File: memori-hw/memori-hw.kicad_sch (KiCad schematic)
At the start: 3 parts, among them J1 Conn_02x04_Odd_Even, J2 Conn_01x07, J3 Conn_01x07

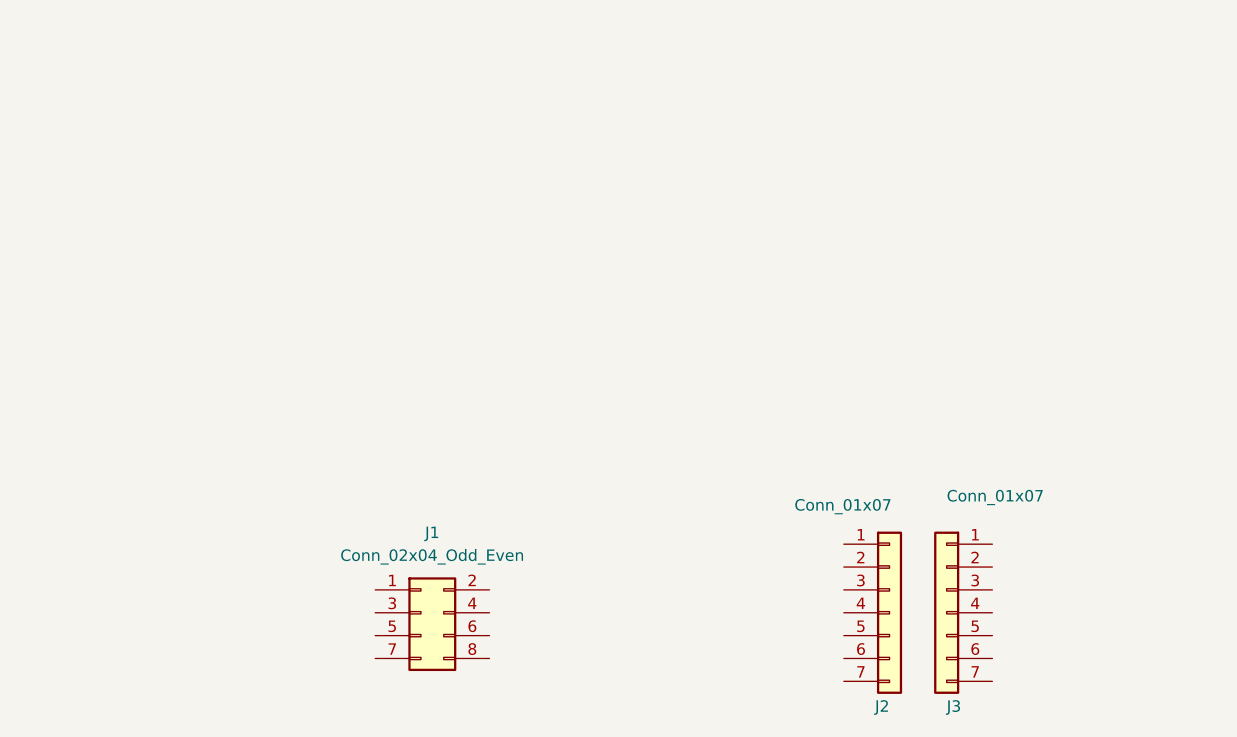
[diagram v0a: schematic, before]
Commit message: feat(hw): Finished with schematic.
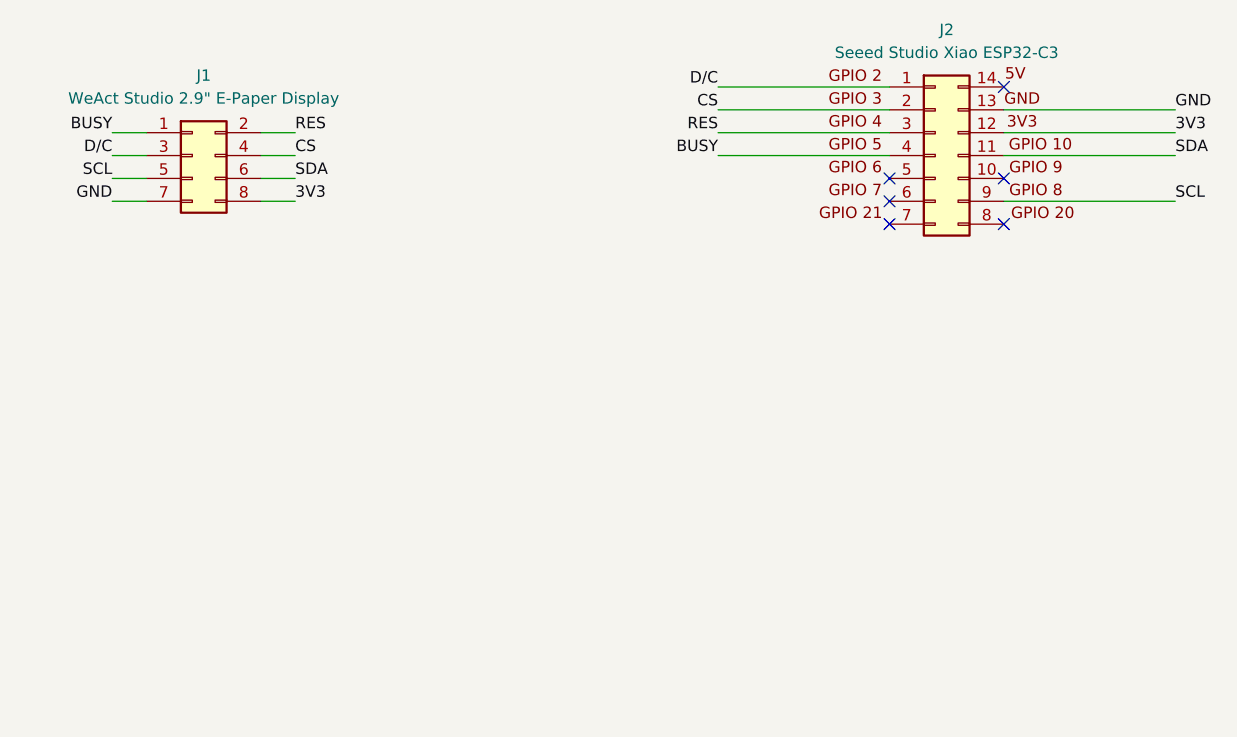
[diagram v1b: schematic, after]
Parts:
- removed J2, J3: Conn_01x07, symbol Connector_Generic:Conn_01x07
- added J2: Seeed Studio Xiao ESP32-C3, Seeed Studio XIAO Series Library:XIAO-ESP32C3-DIP, symbol Connector_Generic:Conn_02x07_Counter_Clockwise
- J1: value Conn_02x04_Odd_Even -> WeAct Studio 2.9{dblquote} E-Paper Display; footprint (none) -> Connector_PinHeader_2.54mm:PinHeader_2x04_P2.54mm_Vertical
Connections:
- net BUSY: now reaches J1.1 (Pin_1)
- net BUSY: now also J2.4 (Pin_4)
- net RES: now reaches J1.2 (Pin_2)
- net RES: now also J2.3 (Pin_3)
- net D/C: now reaches J1.3 (Pin_3)
- net D/C: now also J2.1 (GPIO2)
- net CS: now reaches J1.4 (Pin_4)
- net CS: now also J2.2 (Pin_2)
- net SCL: now reaches J1.5 (Pin_5)
- net SCL: now also J2.9 (Pin_9)
- net SDA: now reaches J1.6 (Pin_6)
- net SDA: now also J2.11 (Pin_11)
- net GND: now reaches J1.7 (Pin_7)
- net GND: now also J2.13 (Pin_13)
- net 3V3: now reaches J1.8 (Pin_8)
- net 3V3: now also J2.12 (Pin_12)
- no-connect marks 0 -> 6
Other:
- title: Mem_C0RE -> MEM_C0RE
- moved on the sheet: J1
